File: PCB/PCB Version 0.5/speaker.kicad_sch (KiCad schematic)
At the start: 4 parts, among them Q1 BSS138

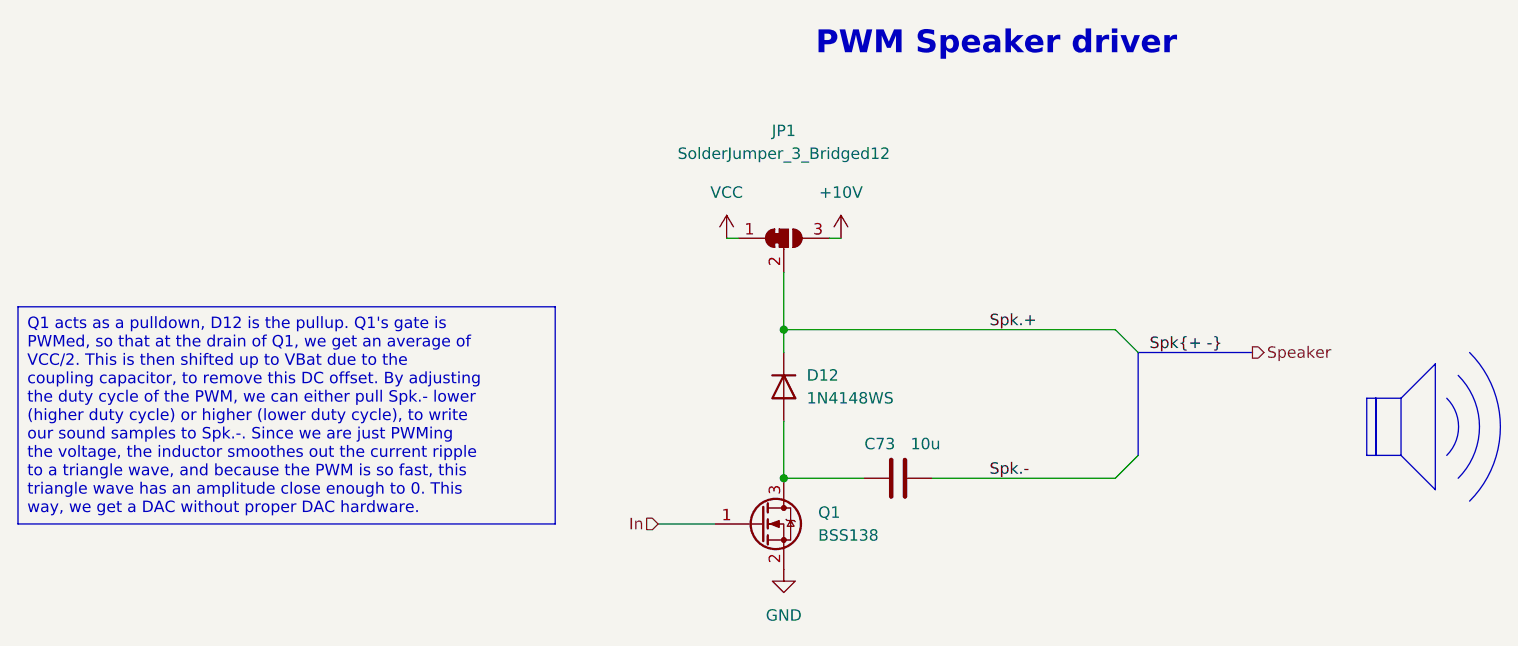
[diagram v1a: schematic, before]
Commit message: schematics nearly done
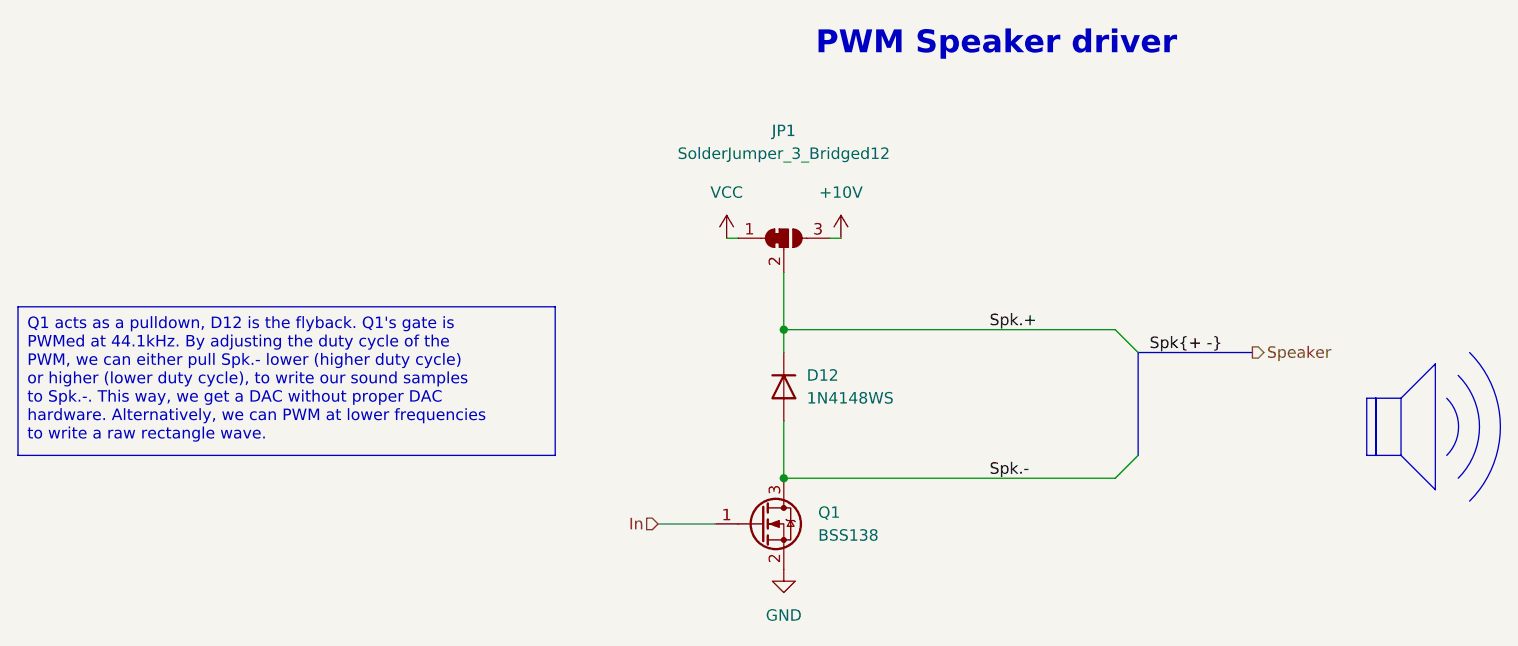
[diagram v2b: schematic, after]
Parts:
- removed C73: 10u, Capacitor_SMD:C_0805_2012Metric, symbol Device:C
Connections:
- net Spk.-: now also D12.2 (A), Q1.3 (D)
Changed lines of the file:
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@@
 	(wire
 		(pts
-			(xy 107.95 80.01) (xy 116.84 80.01)
+			(xy 107.95 80.01) (xy 144.78 80.01)
 		)
 		(stroke
@@
 		(pts
 			(xy 147.32 66.04) (xy 147.32 77.47)
-		)
-		(stroke
-			(width 0)
-			(type default)
-		)
-	)
-	(wire
-		(pts
-			(xy 124.46 80.01) (xy 144.78 80.01)
 		)
 		(stroke
@@
 		)
 	)
-	(text_box "Q1 acts as a pulldown, D12 is the pullup. Q1's gate is PWMed, so that at the drain of Q1, we get an average of VCC/2. This is then shifted up to VBat due to the coupling capacitor, to remove this DC offset. By adjusting the duty cycle of the PWM, we can either pull Spk.- lower (higher duty cycle) or higher (lower duty cycle), to write our sound samples to Spk.-. Since we are just PWMing the voltage, the inductor smoothes out the current ripple to a triangle wave, and because the PWM is so fast, this triangle wave has an amplitude close enough to 0. This way, we get a DAC without proper DAC hardware. "
+	(text_box "Q1 acts as a pulldown, D12 is the flyback. Q1's gate is PWMed at 44.1kHz. By adjusting the duty cycle of the PWM, we can either pull Spk.- lower (higher duty cycle) or higher (lower duty cycle), to write our sound samples to Spk.-. This way, we get a DAC without proper DAC hardware. Alternatively, we can PWM at lower frequencies to write a raw rectangle wave. "
 		(exclude_from_sim no)
 		(at 22.86 60.96 0)
-		(size 59.69 24.13)
+		(size 59.69 16.51)
 		(stroke
 			(width 0)
@@
 	(label "Spk.+"
 		(at 130.81 63.5 0)
-		(fields_autoplaced yes)
 		(effects
 			(font
@@
 	(label "Spk{+ -}"
 		(at 148.59 66.04 0)
-		(fields_autoplaced yes)
 		(effects
 			(font
@@
 	(label "Spk.-"
 		(at 130.81 80.01 0)
-		(fields_autoplaced yes)
 		(effects
 			(font
@@
 		(shape output)
 		(at 160.02 66.04 0)
-		(fields_autoplaced yes)
 		(effects
 			(font
@@
 		(shape input)
 		(at 93.98 85.09 180)
-		(fields_autoplaced yes)
 		(effects
 			(font
@@
 					(unit 1)
 				)
-			)
-		)
-	)
-	(symbol
-		(lib_id "Device:C")
-		(at 120.65 80.01 90)
-		(unit 1)
-		(exclude_from_sim no)
-		(in_bom yes)
-		(on_board yes)
-		(dnp no)
-		(property "Reference" "C73"
-			(at 118.618 76.2 90)
-			(effects
-				(font
-					(size 1.27 1.27)
-				)
-			)
-		)
-		(property "Value" "10u"
-			(at 123.698 76.2 90)
-			(effects
-				(font
-					(size 1.27 1.27)
-				)
-			)
-		)
-		(property "Footprint" "Capacitor_SMD:C_0805_2012Metric"
-			(at 124.46 79.0448 0)
-			(effects
-				(font
-					(size 1.27 1.27)
-				)
-				(hide yes)
-			)
-		)
-		(property "Datasheet" "~"
-			(at 120.65 80.01 0)
-			(effects
-				(font
-					(size 1.27 1.27)
-				)
-				(hide yes)
-			)
-		)
-		(property "Description" "Unpolarized capacitor"
-			(at 120.65 80.01 0)
-			(effects
-				(font
-					(size 1.27 1.27)
-				)
-				(hide yes)
-			)
-		)
-		(pin "2"
-		)
-		(pin "1"
-		)
-		(instances
-			(project ""
-				(path "/1651f454-30c0-48ea-9fcf-6c96a661786a/b926c428-9140-4272-8a94-263799bff176"
-					(reference "C73")
-					(unit 1)
-				)
